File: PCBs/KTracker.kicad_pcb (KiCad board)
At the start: 2 copper layers, 78.5 x 45.7 mm, 44 parts, among them J1 Conn_01x02_Female, J2 Conn_01x04_Female, P1 USB_C_Plug_USB2.0, SW1 Option/FLASH Switch, SW3 SW_SPDT MAIN POWER, U1 ME6211C, U2 TP4056, U4 DW01, U5 FS8205A, U6 ESP-12F, U7 CH340C, U9 MPU-9250

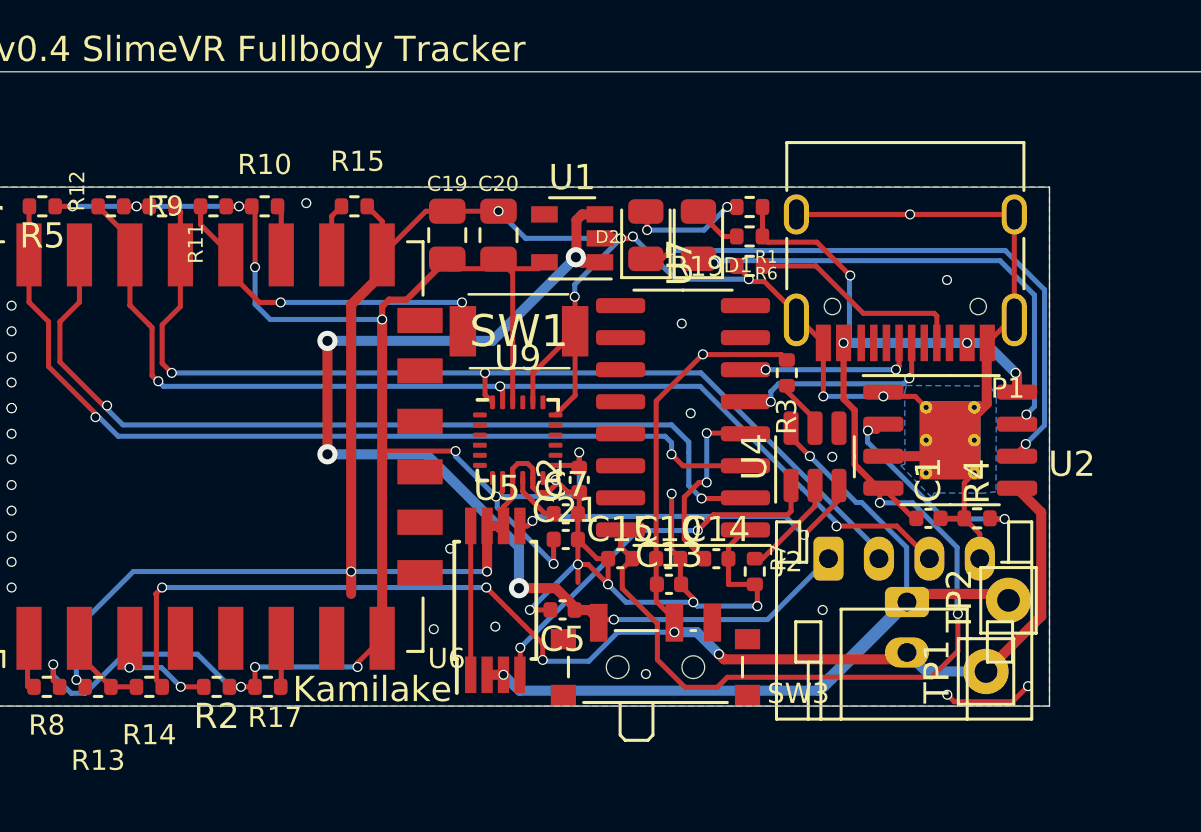
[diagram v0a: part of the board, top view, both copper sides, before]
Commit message: !
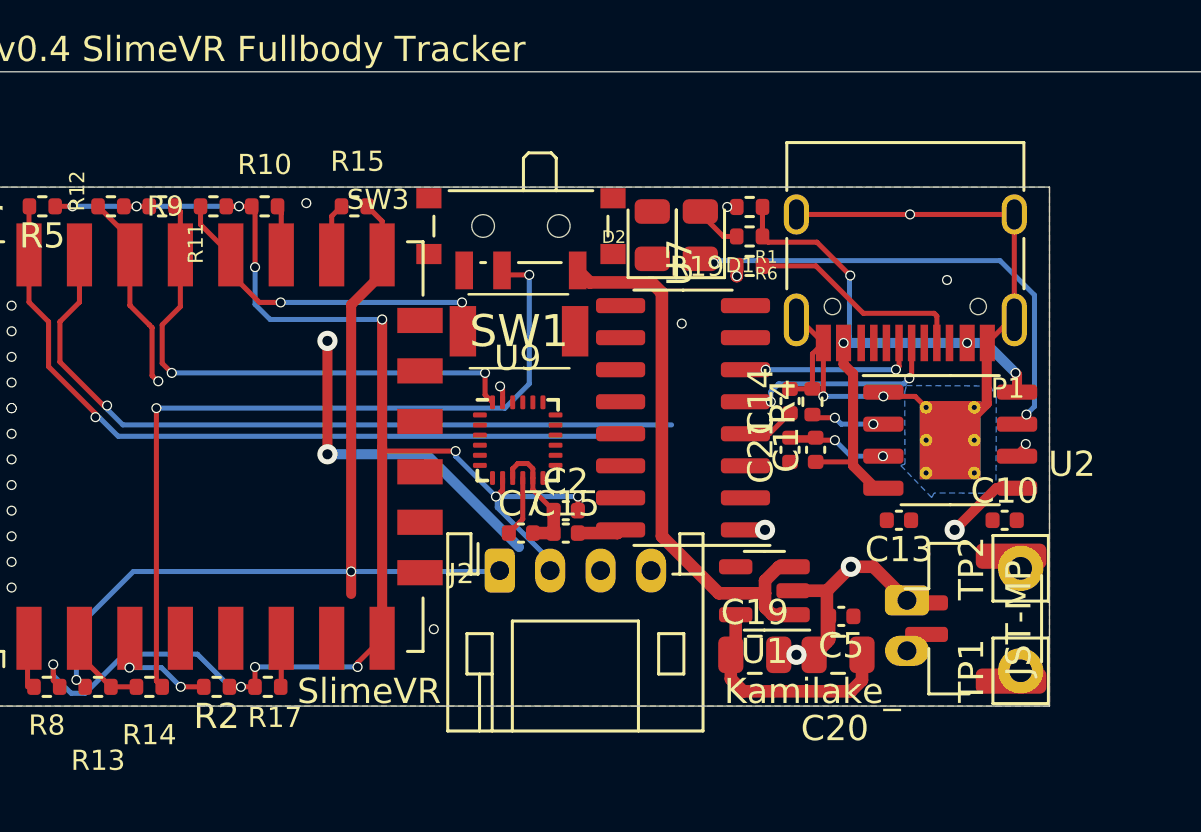
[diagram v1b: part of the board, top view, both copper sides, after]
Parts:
- removed R3: 100R, Resistor_SMD:R_0402_1005Metric
- removed R7: 1K, Resistor_SMD:R_0402_1005Metric
- removed U4: DW01, Package_TO_SOT_SMD:SOT-23-6
- removed U5: FS8205A, Package_SO:TSSOP-8_4.4x3mm_P0.65mm
- added JST-MP: JST_GH_BM02B-GHS-TBT_1x02-1MP_P1.25mm_Vertical, Connector_JST:JST_GH_BM02B-GHS-TBT_1x02-1MP_P1.25mm_Vertical, F.Cu at (136.8, 102.8)
- moved C20 21.4 mm to (131.3, 104.3), turned to 180 degrees
- moved C19 20.6 mm to (128.0, 104.3), turned to 0 degrees
- moved SW3 17.7 mm to (118.7, 87.6), turned to 180 degrees
- moved U1 15.9 mm to (128.4, 101.7)
- moved C10 13.4 mm to (137.9, 98.9)
- moved J2 13.0 mm to (117.9, 100.9)
- moved C5 11.1 mm to (131.4, 102.7)
- moved C21 9.57 mm to (129.4, 96.1), turned to 90 degrees
- moved C13 9.46 mm to (133.7, 98.9), turned to 180 degrees
- moved R4 8.00 mm to (130.3, 94.2), turned to 90 degrees
- moved C14 6.90 mm to (129.4, 94.2), turned to 90 degrees
- moved C1 5.23 mm to (130.4, 96.1), turned to 90 degrees
- moved C15 2.39 mm to (120.5, 99.4)
- moved C7 1.93 mm to (118.7, 99.4)
- moved TP1 1.37 mm to (138.6, 104.9)
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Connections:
- J1 pad 1: BATT- -> GND
- TP2 pad 1: BATT- -> GND
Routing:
- net GND: track 141.6 -> 87.2 mm, vias 43 -> 28
- net BATT-: track 33.9 -> 0.00 mm, vias 2 -> 0
- net SCL: track 42.2 -> 8.61 mm, vias 3 -> 2
- net VBUS: track 54.7 -> 26.1 mm, vias 6 -> 4
- net BATT+: track 63.3 -> 35.0 mm, vias 6 -> 3
- net Net-(D2-Pad1): track 23.6 -> 0.49 mm, vias 2 -> 1
- net SDA: track 40.0 -> 20.9 mm
- net Net-(U4-Pad1): track 15.1 -> 0.00 mm, vias 2 -> 0
- net Net-(U4-Pad3): track 14.3 -> 0.00 mm, vias 2 -> 0
- net VBAT: track 44.9 -> 35.7 mm, vias 5 -> 2
- net +3V3: track 80.1 -> 72.1 mm, vias 13 -> 12
- net Net-(R4-Pad1): track 9.10 -> 2.97 mm
- net Net-(U5-Pad1): track 5.90 -> 0.00 mm
- net Net-(C14-Pad1): track 7.41 -> 2.11 mm, vias 2 -> 0
- net UART_ESP-: track 35.1 -> 29.9 mm, vias 2 -> 1
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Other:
- board text added: "Kamilake_"
- board text added: "SlimeVR"
- board text removed: "Kamilake"
